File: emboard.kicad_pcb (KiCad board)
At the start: 2 copper layers, 85.6 x 54 mm, 4 parts

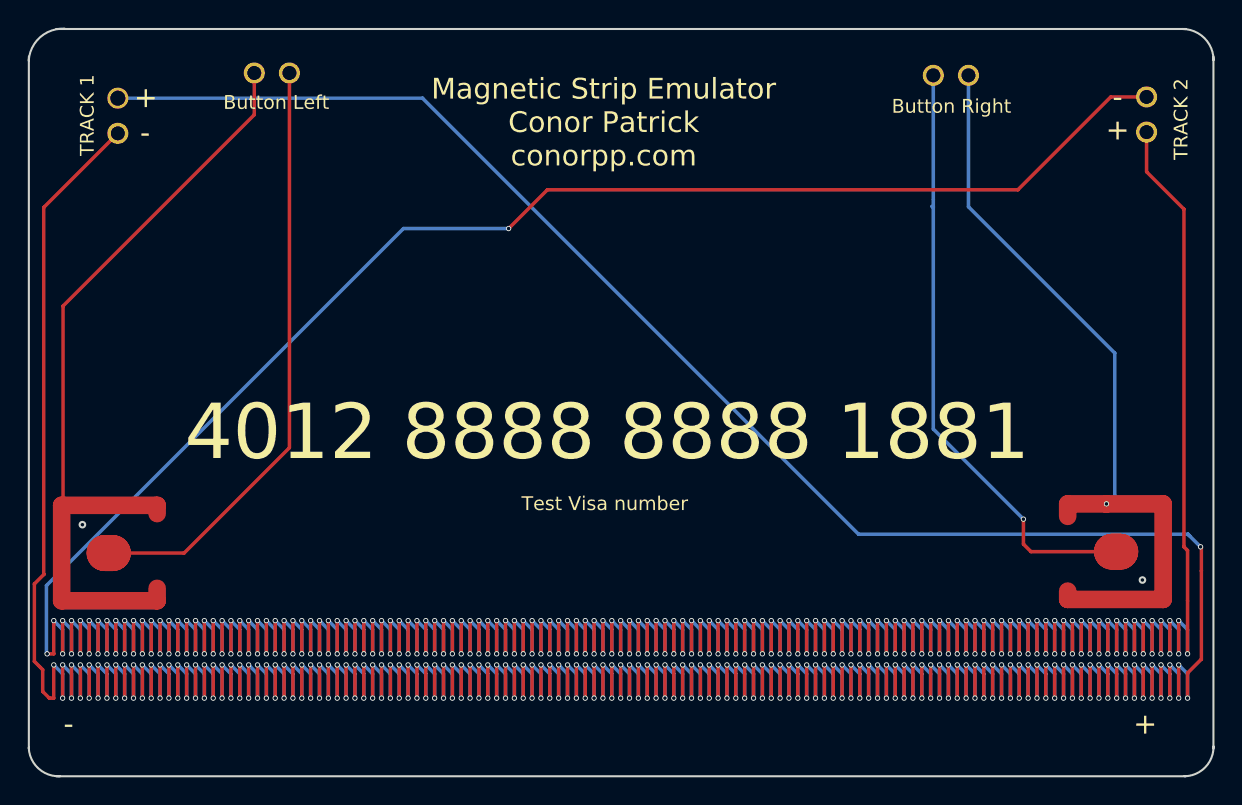
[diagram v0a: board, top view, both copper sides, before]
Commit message: make long ways
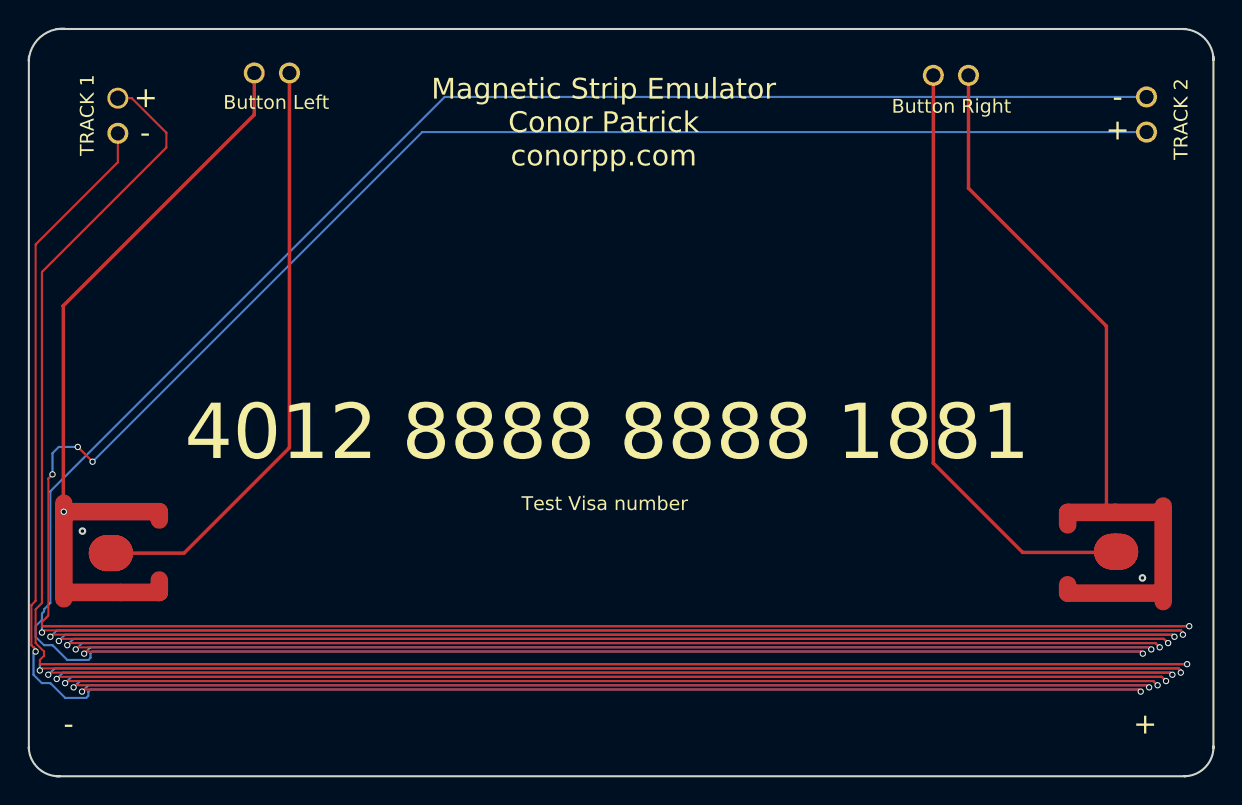
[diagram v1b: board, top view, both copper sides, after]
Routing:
- net (no net): track 0.00 -> 1328.9 mm, vias 0 -> 16
- net -1: track 380.9 -> 1167.9 mm, vias 132 -> 14
- net -2: track 408.6 -> 0.00 mm, vias 124 -> 0
- net +2: track 378.4 -> 0.09 mm, vias 135 -> 1
- net +1: track 414.9 -> 46.2 mm, vias 125 -> 0
- net Buttonleft1: track 44.8 -> 44.0 mm
- net Buttonleft2: track 59.2 -> 59.7 mm, vias 0 -> 1
- net buttonright2: track 44.6 -> 45.1 mm, vias 1 -> 0
- net buttonright1: track 57.8 -> 57.9 mm, vias 1 -> 0
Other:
- outline, holes or cut-outs redrawn
